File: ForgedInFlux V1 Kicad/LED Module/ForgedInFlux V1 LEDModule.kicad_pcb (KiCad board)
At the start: 2 copper layers, 59.6 x 99.6 mm, 0 parts

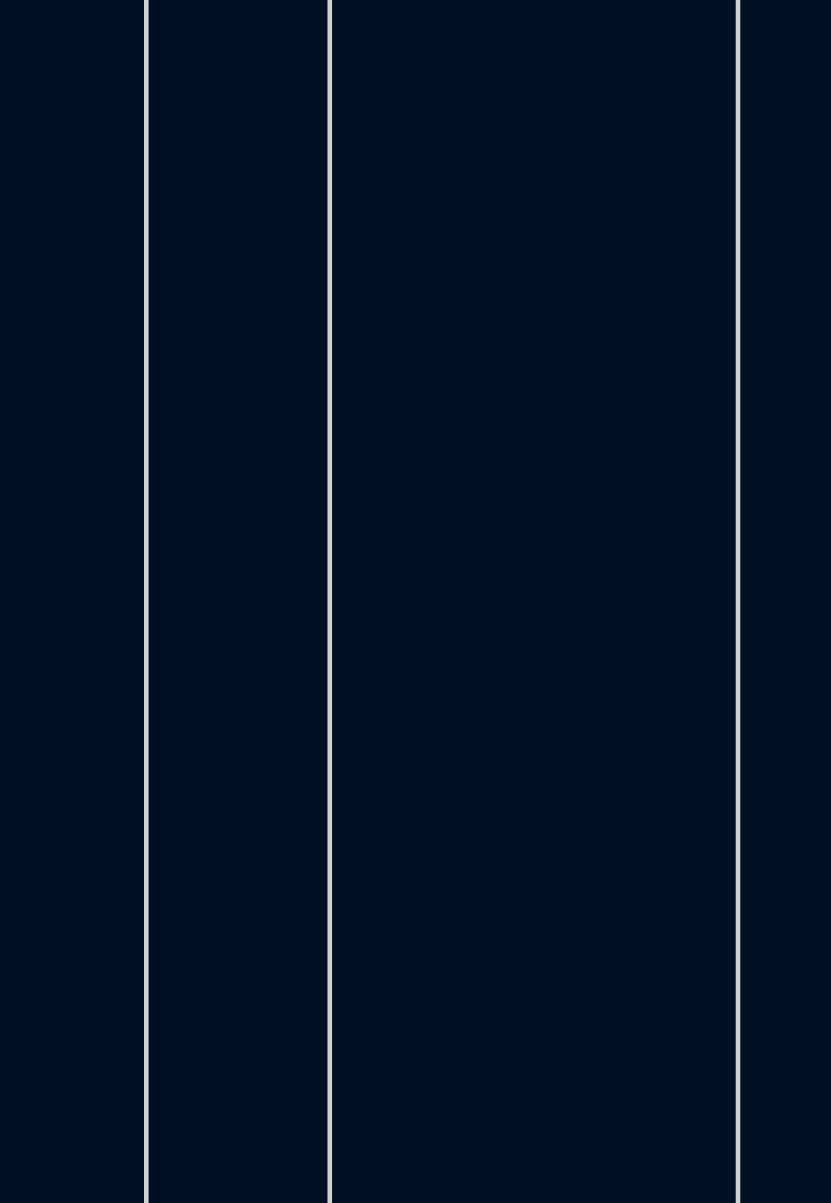
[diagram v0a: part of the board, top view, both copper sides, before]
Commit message: Edited Schematic
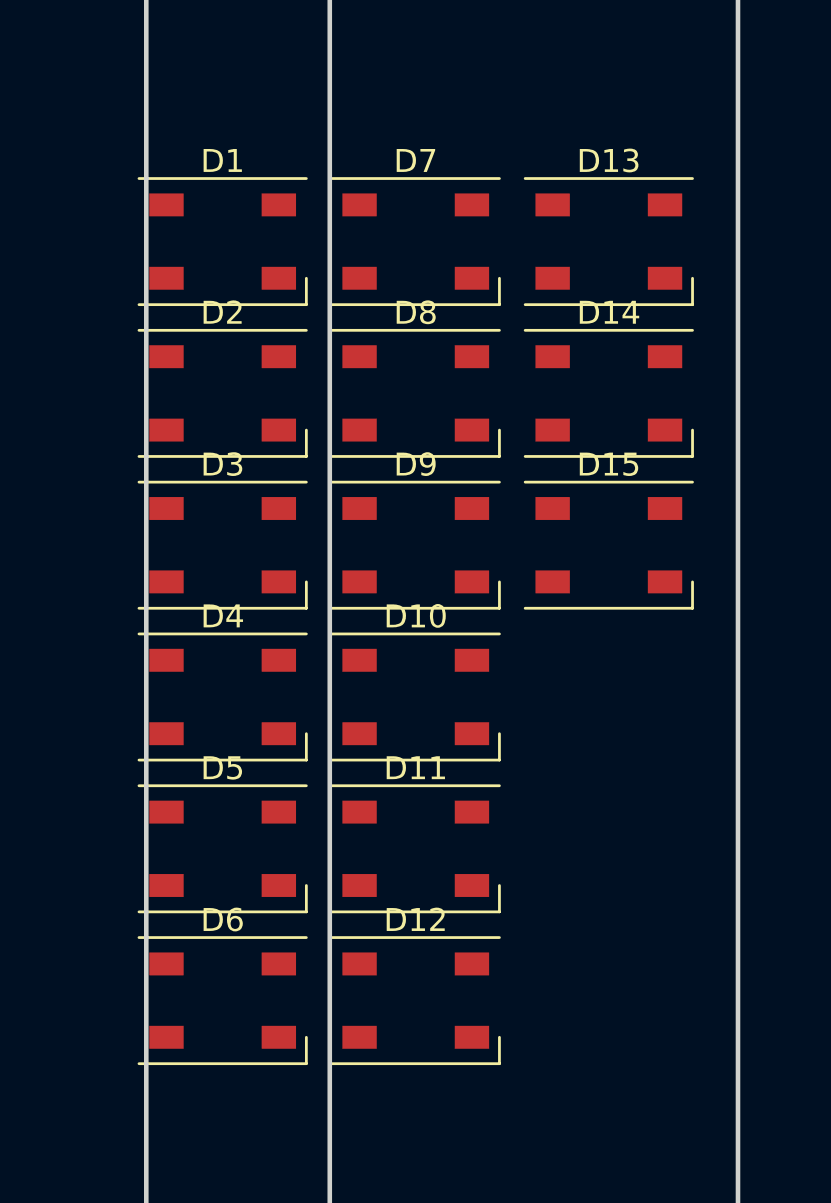
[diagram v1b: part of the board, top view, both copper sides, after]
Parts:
- added D1: SK6812, LED_SMD:LED_SK6812_PLCC4_5.0x5.0mm_P3.2mm, F.Cu at (49.1, 56.3)
- added D10: SK6812, LED_SMD:LED_SK6812_PLCC4_5.0x5.0mm_P3.2mm, F.Cu at (57.5, 76.2)
- added D11: SK6812, LED_SMD:LED_SK6812_PLCC4_5.0x5.0mm_P3.2mm, F.Cu at (57.5, 82.8)
- added D12: SK6812, LED_SMD:LED_SK6812_PLCC4_5.0x5.0mm_P3.2mm, F.Cu at (57.5, 89.4)
- added D13: SK6812, LED_SMD:LED_SK6812_PLCC4_5.0x5.0mm_P3.2mm, F.Cu at (66.0, 56.3)
- added D14: SK6812, LED_SMD:LED_SK6812_PLCC4_5.0x5.0mm_P3.2mm, F.Cu at (66.0, 62.9)
- added D15: SK6812, LED_SMD:LED_SK6812_PLCC4_5.0x5.0mm_P3.2mm, F.Cu at (66.0, 69.5)
- added D2: SK6812, LED_SMD:LED_SK6812_PLCC4_5.0x5.0mm_P3.2mm, F.Cu at (49.1, 62.9)
- added D3: SK6812, LED_SMD:LED_SK6812_PLCC4_5.0x5.0mm_P3.2mm, F.Cu at (49.1, 69.5)
- added D4: SK6812, LED_SMD:LED_SK6812_PLCC4_5.0x5.0mm_P3.2mm, F.Cu at (49.1, 76.2)
- added D5: SK6812, LED_SMD:LED_SK6812_PLCC4_5.0x5.0mm_P3.2mm, F.Cu at (49.1, 82.8)
- added D6: SK6812, LED_SMD:LED_SK6812_PLCC4_5.0x5.0mm_P3.2mm, F.Cu at (49.1, 89.4)
- added D7: SK6812, LED_SMD:LED_SK6812_PLCC4_5.0x5.0mm_P3.2mm, F.Cu at (57.5, 56.3)
- added D8: SK6812, LED_SMD:LED_SK6812_PLCC4_5.0x5.0mm_P3.2mm, F.Cu at (57.5, 62.9)
- added D9: SK6812, LED_SMD:LED_SK6812_PLCC4_5.0x5.0mm_P3.2mm, F.Cu at (57.5, 69.5)
